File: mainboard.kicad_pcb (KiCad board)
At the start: 2 copper layers, 57.1 x 30 mm, 26 parts, among them J1 105017-1001, J2 Conn_01x04_Female, J3 Conn_01x02_Female, J4 Conn_01x09_Female, J5 Conn_01x02_Female, J6 Conn_01x02_Female, J7 Conn_01x04_Female, Q1 AOD4184A, U1 ESP32-WROOM-32E_(16MB), U3 AMS1117-3.3, U4 PAM8403DR

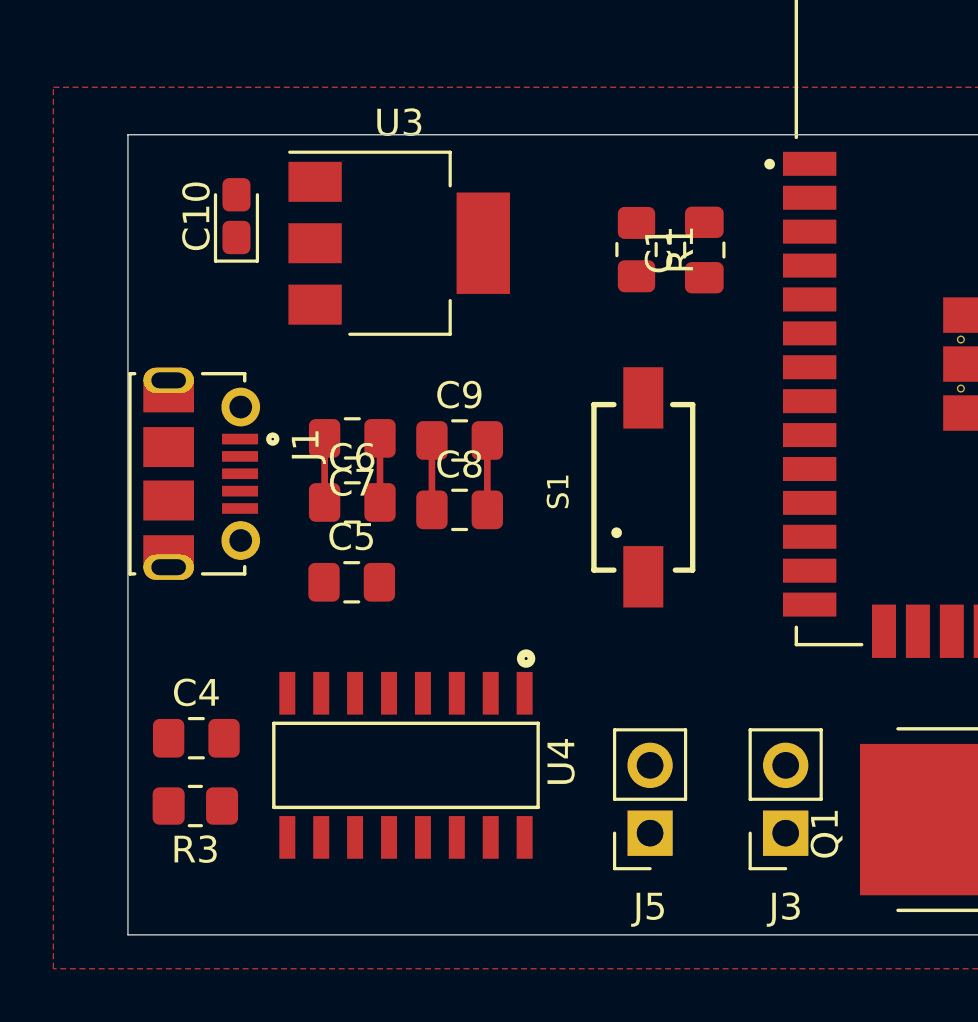
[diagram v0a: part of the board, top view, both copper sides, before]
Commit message: beetje tracing gedaan
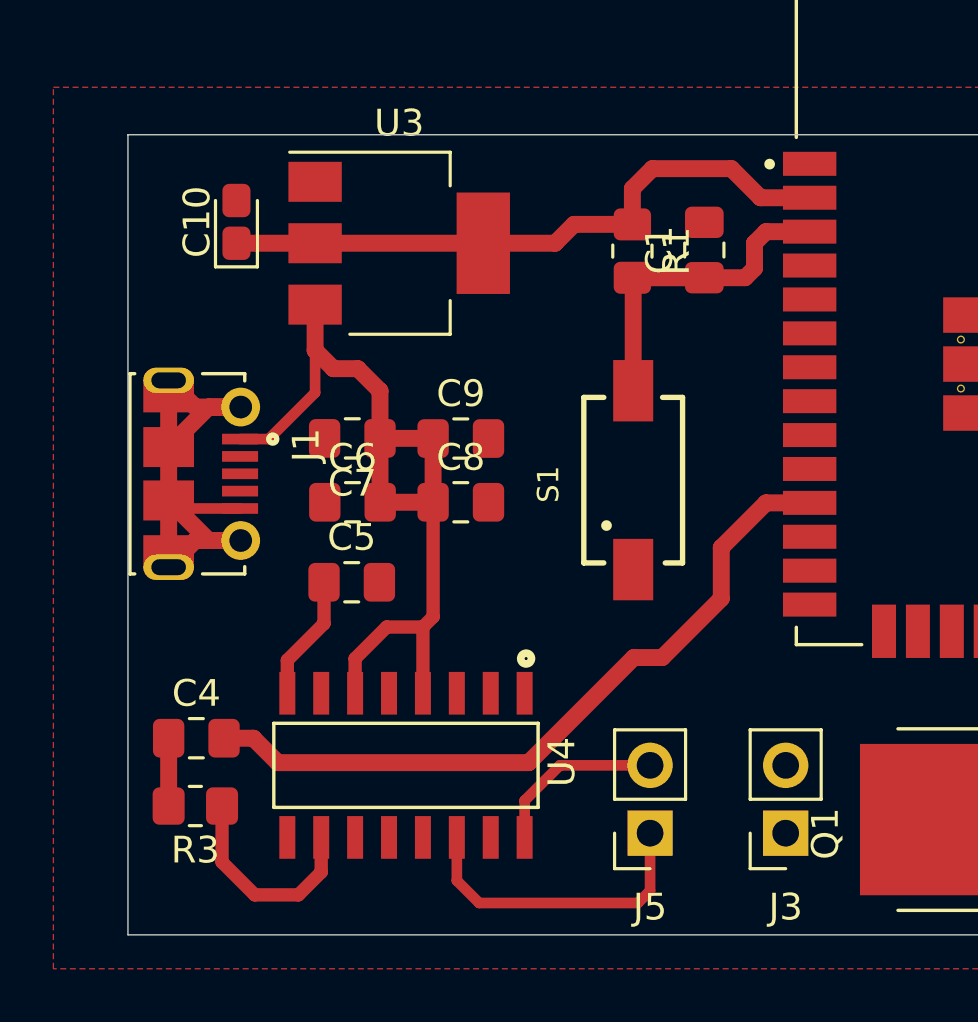
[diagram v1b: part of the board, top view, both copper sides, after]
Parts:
- moved S1 0.46 mm to (98.9, 96.3)
- moved C8 0.29 mm to (92.5, 97.1)
- moved C10 0.22 mm to (84.1, 86.6)
- moved R1 0.16 mm to (98.9, 87.7)
- moved C9 0.08 mm to (92.5, 94.7)
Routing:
- net 5V: track 5.00 -> 33.9 mm
- net INR: track 0.00 -> 27.5 mm
- net 3V3: track 0.00 -> 23.9 mm
- net GND: track 5.00 -> 22.7 mm
- net Net-(C1-Pad1): track 0.00 -> 12.2 mm
- net -OUT_R: track 0.00 -> 11.6 mm
- net Net-(R3-Pad1): track 0.00 -> 7.98 mm
- net +OUT_R: track 0.00 -> 6.63 mm
- net Net-(C5-Pad1): track 0.00 -> 4.73 mm
- net Net-(C4-Pad1): track 0.00 -> 2.54 mm

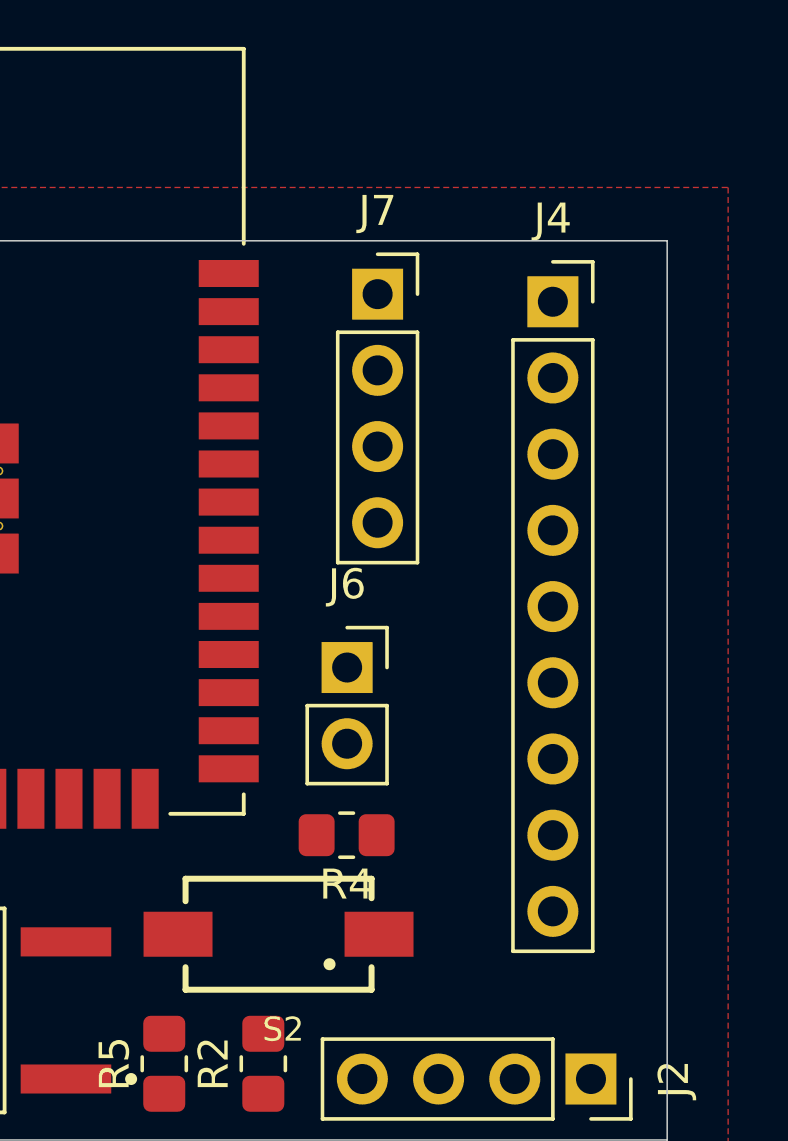
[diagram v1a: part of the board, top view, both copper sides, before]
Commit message: sorry stef pt. 3
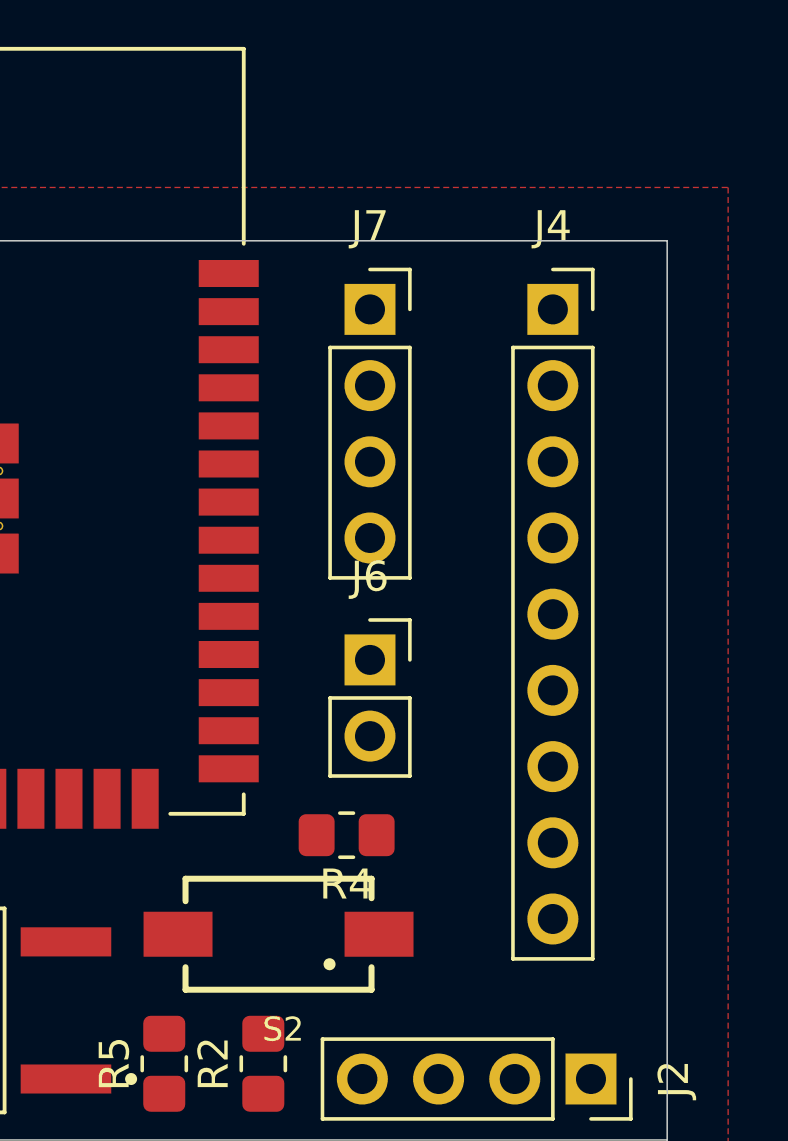
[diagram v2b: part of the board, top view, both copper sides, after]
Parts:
- moved J6 0.80 mm to (127.3, 97.3)
- moved J7 0.57 mm to (127.3, 85.6)
- moved J4 0.25 mm to (133.3, 85.6)

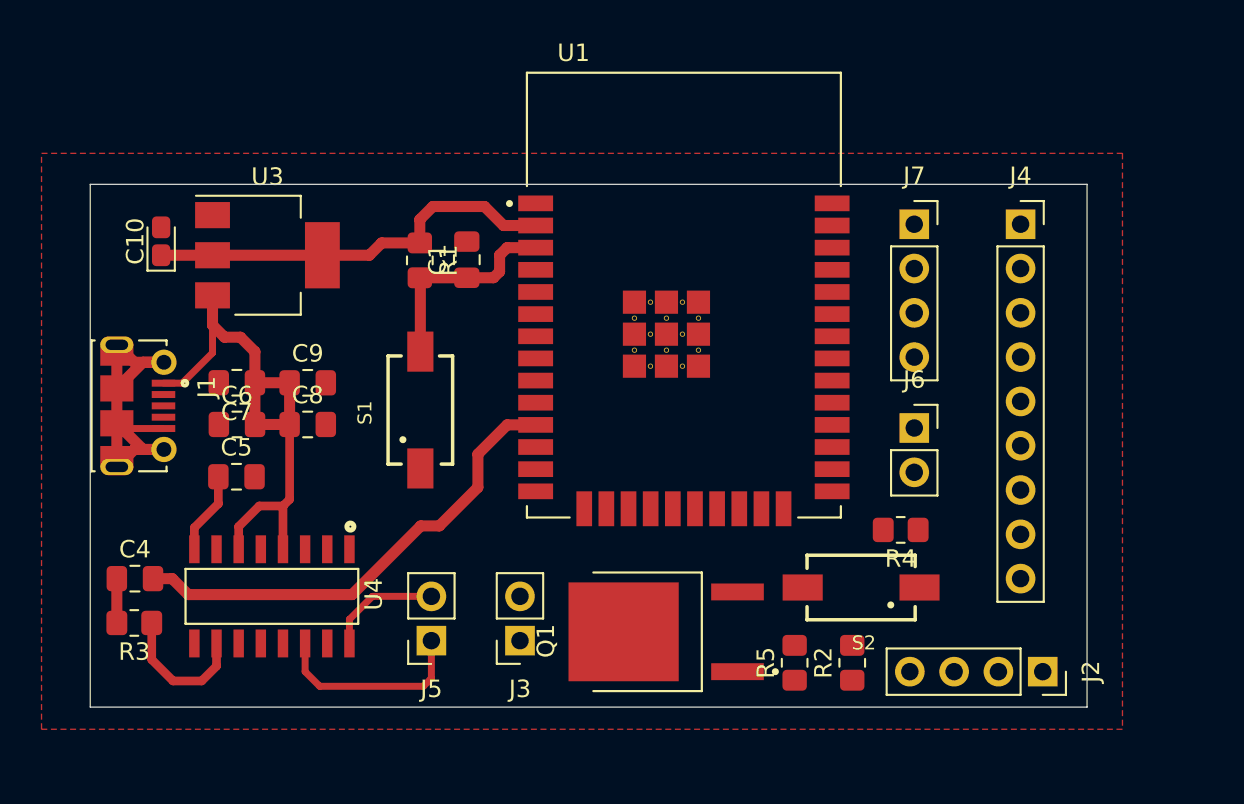
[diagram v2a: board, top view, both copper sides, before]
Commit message: tis fokking mooi wtf
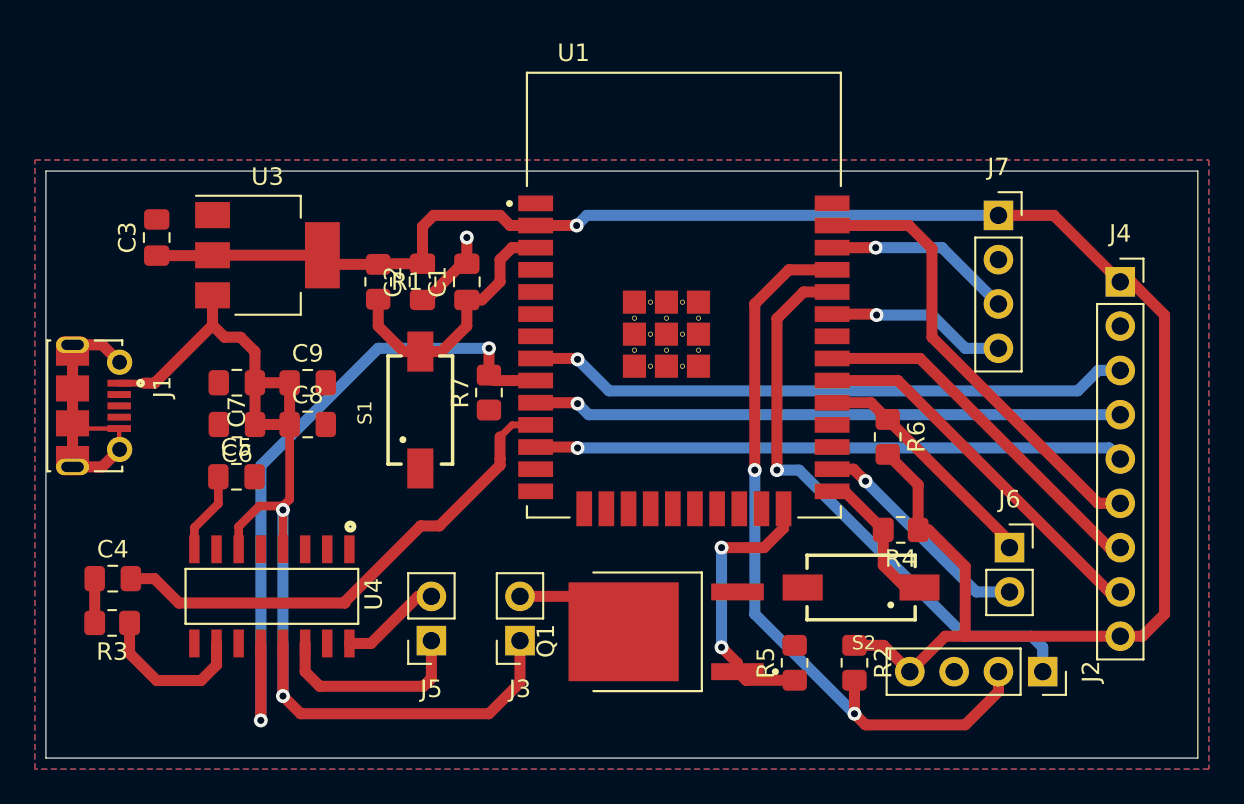
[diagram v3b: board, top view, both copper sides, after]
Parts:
- removed C10: CP, Capacitor_Tantalum_SMD:CP_EIA-1608-08_AVX-J_Pad1.25x1.05mm_HandSolder
- added C2: 100n, Capacitor_SMD:C_0805_2012Metric_Pad1.18x1.45mm_HandSolder, F.Cu at (99.1, 88.9)
- added C3: 22u, Capacitor_SMD:C_0805_2012Metric_Pad1.18x1.45mm_HandSolder, F.Cu at (83.8, 86.4)
- added R6: 10K, Resistor_SMD:R_0805_2012Metric_Pad1.20x1.40mm_HandSolder, F.Cu at (125.7, 97.8)
- added R7: 10K, Resistor_SMD:R_0805_2012Metric_Pad1.20x1.40mm_HandSolder, F.Cu at (102.9, 95.2)
- C1: value C -> 100n
- C4: value C -> 0.47u
- C5: value C -> 0.1u
- C6, C7, C9: value C -> 1u
- C8: value C -> 470u
- R1, R2, R3, R4, R5: value R -> 10K
- moved J6 8.77 mm to (132.7, 104.1)
- moved J4 6.60 mm to (139.1, 88.9)
- moved J7 4.85 mm to (132.1, 85.1)
- moved R1 2.68 mm to (96.5, 88.9)
- moved J1 2.54 mm to (79.0, 96.0)
- moved C1 1.27 mm to (101.6, 88.9)
- moved R3 1.27 mm to (81.3, 108.5)
- moved C4 1.27 mm to (81.3, 105.9)
- moved R2 0.13 mm to (123.8, 110.7), turned to 270 degrees
- turned C6 to 180 degrees
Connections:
- C6 pad 1: GND -> 5V
- C6 pad 2: 5V -> GND
- J4 pad 3: TFT_CS -> TFT_RST
- J4 pad 4: TFT_RST -> TFT_CS
- J4 pad 7: TFT_CLK -> TFT_MISO
- J4 pad 8: 3V3 -> TFT_CLK
- J4 pad 9: TFT_MISO -> 3V3
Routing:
- net 3V3: track 23.9 -> 112.9 mm, vias 0 -> 1
- net TXD: track 0.00 -> 43.5 mm, vias 0 -> 2
- net SHND: track 0.00 -> 39.2 mm, vias 0 -> 2
- net TFT_RST: track 0.00 -> 35.3 mm, vias 0 -> 1
- net TFT_DC: track 0.00 -> 33.8 mm, vias 0 -> 1
- net TFT_CS: track 0.00 -> 33.8 mm, vias 0 -> 1
- net RXD: track 0.00 -> 33.3 mm, vias 0 -> 1
- net 5V: track 33.9 -> 64.6 mm, vias 0 -> 2
- net TFT_MOSI: track 0.00 -> 26.1 mm
- net TFT_CLK: track 0.00 -> 21.5 mm
- net TFT_MISO: track 0.00 -> 21.0 mm
- net Mosfet_Trig: track 0.00 -> 16.1 mm, vias 0 -> 2
- net PN532_RESET: track 0.00 -> 13.8 mm
- net PN532_IRQ: track 0.00 -> 13.1 mm, vias 0 -> 1
- net SCL: track 0.00 -> 10.9 mm, vias 0 -> 1
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- added copper zone on F.Cu, net (none)
- added copper zone on B.Cu, net GND
- removed copper zone on F.Cu, net GND
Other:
- board size 57.1 x 30 mm -> 66 x 33.7 mm
